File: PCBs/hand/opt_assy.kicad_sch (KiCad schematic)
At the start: 1 part

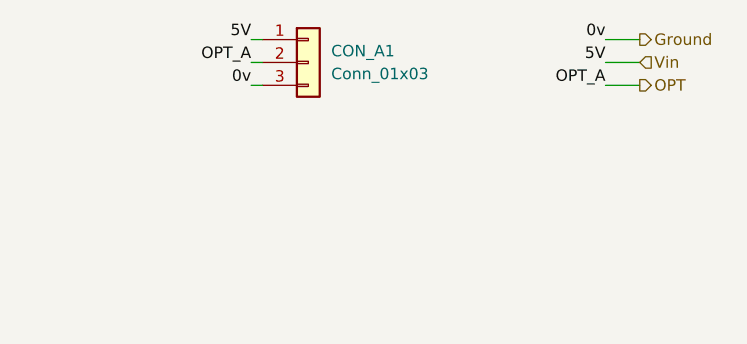
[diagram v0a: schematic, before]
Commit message: Added pcb pdfs
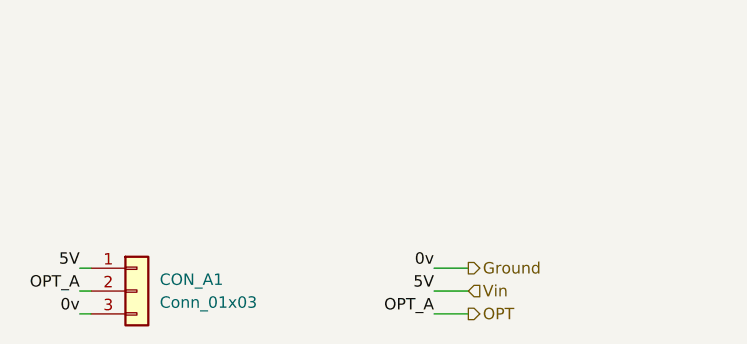
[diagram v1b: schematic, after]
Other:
- moved on the sheet: CON_A1
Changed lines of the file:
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@@
 (kicad_sch (version 20230121) (generator eeschema)
   (paper "A5")
-  (wire (pts (xy 100.33 39.37) (xy 101.6 39.37))
+  (wire (pts (xy 81.28 64.77) (xy 82.55 64.77))
     (stroke (width 0) (type default))
   )
-  (wire (pts (xy 139.7 44.45) (xy 143.51 44.45))
+  (wire (pts (xy 120.65 69.85) (xy 124.46 69.85))
     (stroke (width 0) (type default))
   )
-  (wire (pts (xy 100.33 41.91) (xy 101.6 41.91))
+  (wire (pts (xy 81.28 67.31) (xy 82.55 67.31))
     (stroke (width 0) (type default))
   )
-  (wire (pts (xy 139.7 39.37) (xy 143.51 39.37))
+  (wire (pts (xy 120.65 64.77) (xy 124.46 64.77))
     (stroke (width 0) (type default))
   )
-  (wire (pts (xy 139.7 41.91) (xy 143.51 41.91))
+  (wire (pts (xy 120.65 67.31) (xy 124.46 67.31))
     (stroke (width 0) (type default))
   )
-  (wire (pts (xy 100.33 44.45) (xy 101.6 44.45))
+  (wire (pts (xy 81.28 69.85) (xy 82.55 69.85))
     (stroke (width 0) (type default))
   )
-  (label "0v" (at 100.33 44.45 180) (fields_autoplaced)
+  (label "0v" (at 81.28 69.85 180) (fields_autoplaced)
     (effects (font (size 1.27 1.27)) (justify right bottom))
   )
-  (label "OPT_A" (at 100.33 41.91 180) (fields_autoplaced)
+  (label "OPT_A" (at 81.28 67.31 180) (fields_autoplaced)
     (effects (font (size 1.27 1.27)) (justify right bottom))
   )
-  (label "5V" (at 139.7 41.91 180) (fields_autoplaced)
+  (label "5V" (at 120.65 67.31 180) (fields_autoplaced)
     (effects (font (size 1.27 1.27)) (justify right bottom))
   )
-  (label "5V" (at 100.33 39.37 180) (fields_autoplaced)
+  (label "5V" (at 81.28 64.77 180) (fields_autoplaced)
     (effects (font (size 1.27 1.27)) (justify right bottom))
   )
-  (label "OPT_A" (at 139.7 44.45 180) (fields_autoplaced)
+  (label "OPT_A" (at 120.65 69.85 180) (fields_autoplaced)
     (effects (font (size 1.27 1.27)) (justify right bottom))
   )
-  (label "0v" (at 139.7 39.37 180) (fields_autoplaced)
+  (label "0v" (at 120.65 64.77 180) (fields_autoplaced)
     (effects (font (size 1.27 1.27)) (justify right bottom))
   )
-  (hierarchical_label "Ground" (shape output) (at 143.51 39.37 0) (fields_autoplaced)
+  (hierarchical_label "Ground" (shape output) (at 124.46 64.77 0) (fields_autoplaced)
     (effects (font (size 1.27 1.27)) (justify left))
   )
-  (hierarchical_label "OPT" (shape output) (at 143.51 44.45 0) (fields_autoplaced)
+  (hierarchical_label "OPT" (shape output) (at 124.46 69.85 0) (fields_autoplaced)
     (effects (font (size 1.27 1.27)) (justify left))
   )
-  (hierarchical_label "Vin" (shape input) (at 143.51 41.91 0) (fields_autoplaced)
+  (hierarchical_label "Vin" (shape input) (at 124.46 67.31 0) (fields_autoplaced)
     (effects (font (size 1.27 1.27)) (justify left))
   )
-  (symbol (lib_id "Connector_Generic:Conn_01x03") (at 106.68 41.91 0) (unit 1)
+  (symbol (lib_id "Connector_Generic:Conn_01x03") (at 87.63 67.31 0) (unit 1)
     (in_bom yes) (on_board yes) (dnp no) (fields_autoplaced)
-    (property "Reference" "CON_A1" (at 109.22 40.64 0)
+    (property "Reference" "CON_A1" (at 90.17 66.04 0)
       (effects (font (size 1.27 1.27)) (justify left))
     )
-    (property "Value" "Conn_01x03" (at 109.22 43.18 0)
+    (property "Value" "Conn_01x03" (at 90.17 68.58 0)
       (effects (font (size 1.27 1.27)) (justify left))
     )
-    (property "Footprint" "Connector_PinHeader_2.54mm:PinHeader_1x03_P2.54mm_Vertical" (at 106.68 41.91 0)
+    (property "Footprint" "Connector_PinHeader_2.54mm:PinHeader_1x03_P2.54mm_Vertical" (at 87.63 67.31 0)
       (effects (font (size 1.27 1.27)) hide)
     )
-    (property "Datasheet" "~" (at 106.68 41.91 0)
+    (property "Datasheet" "~" (at 87.63 67.31 0)
       (effects (font (size 1.27 1.27)) hide)
     )
@@
     (instances
       (project "hand"
-        (path "/5df167e9-440d-40dc-8690-43ffe4e4c50d"
-          (reference "CON_A1") (unit 1)
-        )
         (path "/5df167e9-440d-40dc-8690-43ffe4e4c50d/0c4cb80d-a6d8-4cad-aec7-41b1541506df"
           (reference "CON_A1") (unit 1)
